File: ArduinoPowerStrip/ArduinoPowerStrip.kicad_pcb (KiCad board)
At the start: 2 copper layers, 53.3 x 68.5 mm, 15 parts, among them P101 Triac1, P102 Triac1, Q101 Q_NPN_BEC, Q102 Q_NPN_BEC, U101 MOC3041M, U102 MOC3041M, U103 TRIAC, U104 TRIAC

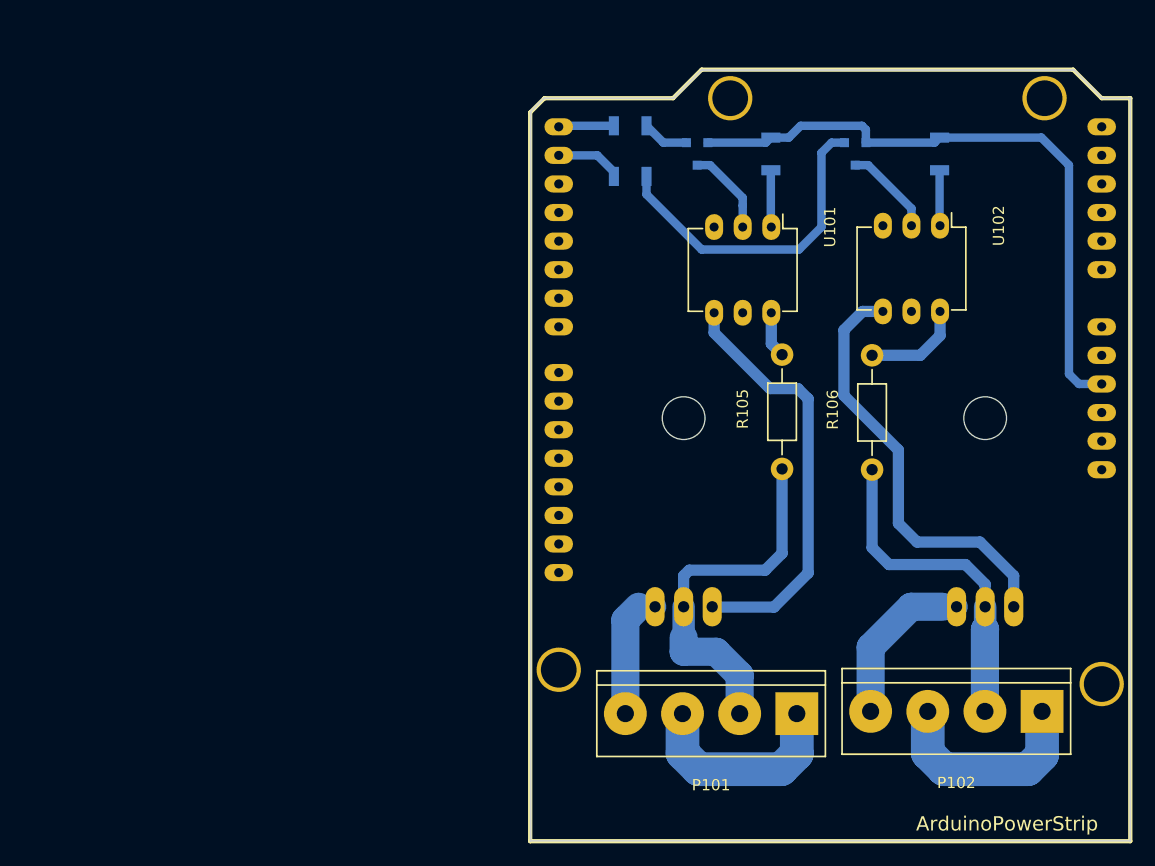
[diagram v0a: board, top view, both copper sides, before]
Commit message: Initial draft of the final board
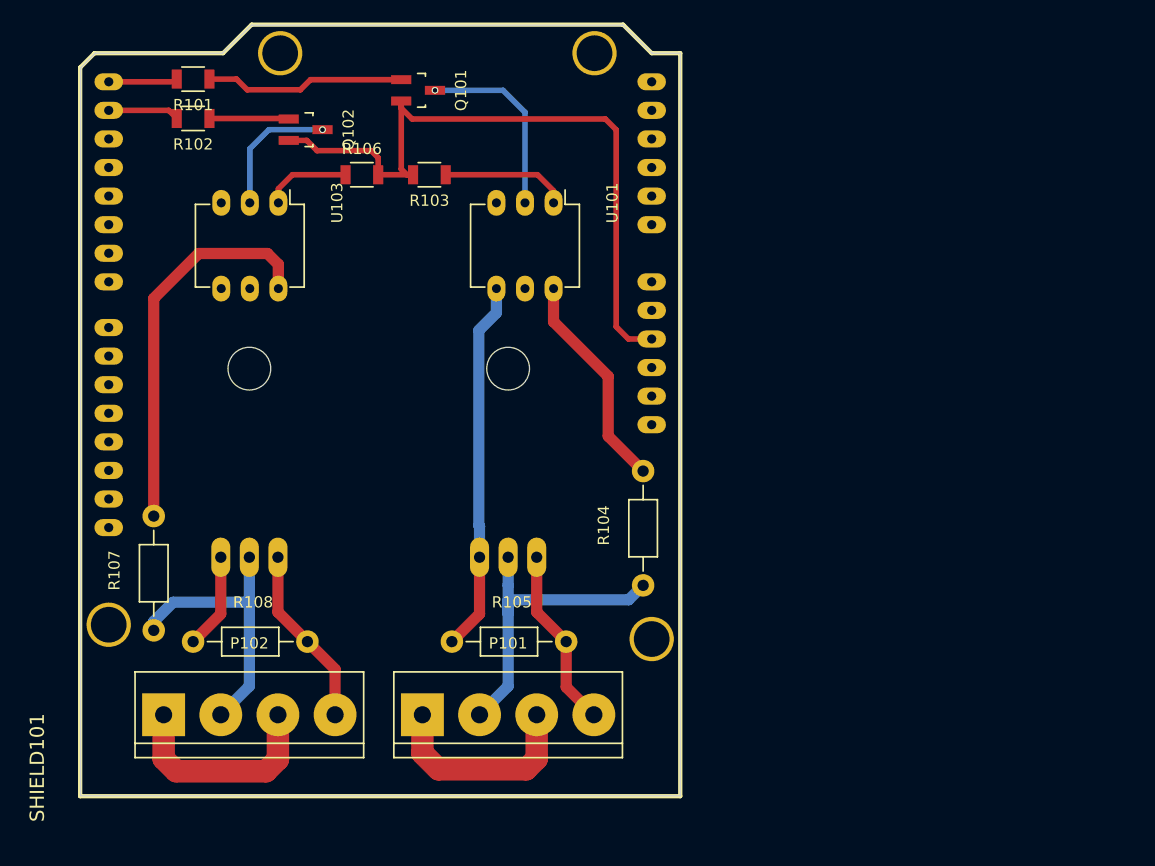
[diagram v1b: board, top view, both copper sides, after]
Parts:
- removed ArduinoPowerStrip: ARDUINO_SHIELD, ArduinoShield:ArduinoShield
- added R107: 361, Resistors_ThroughHole:Resistor_Horizontal_RM10mm, F.Cu at (76.5, 101.5)
- added R108: 331, Resistors_ThroughHole:Resistor_Horizontal_RM10mm, F.Cu at (80.0, 102.5)
- added SHIELD101: ARDUINO_SHIELD, ArduinoShield:ArduinoShield, F.Cu at (123.3, 116.2)
- P101: value Triac1 -> Con1
- P102: value Triac1 -> Con2
- Q101, Q102: value Q_NPN_BEC -> BC847-SOT23; footprint TO_SOT_Packages_SMD:SOT-23 -> TO_SOT_Packages_SMD:SOT-23_Handsoldering; moved to F.Cu
- R101, R102: value R_Small -> 331; moved to F.Cu
- R103: value R_Small -> 131; moved to F.Cu
- R104: value R_Small -> 361; footprint Resistors_SMD:R_1206 -> Resistors_ThroughHole:Resistor_Horizontal_RM10mm; moved to F.Cu
- R105: value R_Small -> 331
- R106: value R_Small -> 131; footprint Resistors_ThroughHole:Resistor_Horizontal_RM10mm -> Resistors_SMD:R_1206
- U102: value MOC3041M -> BTA06-600BW; footprint Housings_DIP:DIP-6_W7.62mm_LongPads -> TO_SOT_Packages_THT:TO-220_Neutral123_Horizontal_LargePads; moved to B.Cu
- U103: value TRIAC -> MOC3041M; footprint TO_SOT_Packages_THT:TO-220_Neutral123_Horizontal_Reverse_LargePads -> Housings_DIP:DIP-6_W7.62mm_LongPads; moved to F.Cu
- U104: value TRIAC -> BTA06-600BW; footprint TO_SOT_Packages_THT:TO-220_Neutral123_Horizontal_Reverse_LargePads -> TO_SOT_Packages_THT:TO-220_Neutral123_Horizontal_LargePads
- moved U104 65.5 mm to (85.0, 95.0)
- moved P102 62.8 mm to (85.0, 109.0), turned to 0 degrees
- moved R106 52.4 mm to (95.0, 61.0), turned to 0 degrees
- moved U103 50.9 mm to (87.6, 63.5), turned to 270 degrees
- moved Q102 48.9 mm to (90.0, 57.0), turned to 270 degrees
- moved U102 48.4 mm to (108.0, 95.0), turned to 180 degrees
- moved R104 46.5 mm to (120.0, 97.5)
- moved R102 39.2 mm to (80.0, 56.0)
- moved R101 39.1 mm to (80.0, 52.5)
- moved R105 33.1 mm to (103.0, 102.5), turned to 0 degrees
- moved R103 30.4 mm to (101.0, 61.0), turned to 180 degrees
- moved Q101 25.4 mm to (100.0, 53.5), turned to 270 degrees
- moved U101 19.5 mm to (112.0, 63.5)
- moved P101 18.0 mm to (108.0, 109.0), turned to 0 degrees
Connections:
- R104 pad 1: Net-(R104-Pad1) -> /Triac1L
- R104 pad 2: /Gnd -> Net-(R104-Pad2)
- R105 pad 1: /Triac1L -> Net-(R105-Pad1)
- R105 pad 2: Net-(R105-Pad2) -> /Triac1O
- R106 pad 1: /Triac2L -> Net-(R106-Pad1)
- R106 pad 2: Net-(R106-Pad2) -> /Gnd
- U101 pad 4: Net-(U101-Pad4) -> Net-(R105-Pad1)
- U101 pad 6: Net-(R105-Pad2) -> Net-(R104-Pad2)
- U102 pad 1: Net-(R104-Pad1) -> /Triac1O
- U102 pad 2: /Q2Out -> /Triac1L
- U102 pad 3: (no net) -> Net-(R105-Pad1)
- U103 pad 1: /Triac1O -> Net-(R106-Pad1)
- U103 pad 2: /Triac1L -> /Q2Out
- U103 pad 3: Net-(U101-Pad4) -> (no net)
- U104 pad 3: Net-(U102-Pad4) -> Net-(R108-Pad1)
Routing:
- net Net-(U102-Pad4): track 38.3 -> 0.00 mm
- net Net-(U101-Pad4): track 37.9 -> 0.00 mm
- net Net-(R107-Pad2): track 0.00 -> 34.6 mm
- net Net-(R105-Pad1): track 0.00 -> 34.0 mm
- net Net-(Q102-Pad1): track 29.0 -> 7.07 mm
- net Net-(R104-Pad2): track 0.00 -> 19.5 mm
- net Net-(Q101-Pad1): track 4.17 -> 17.8 mm
- net /Q1Out: track 7.85 -> 17.2 mm, vias 0 -> 1
- net Net-(R106-Pad2): track 8.91 -> 0.00 mm
- net Net-(R108-Pad1): track 0.00 -> 8.52 mm
- net Net-(R106-Pad1): track 0.00 -> 7.74 mm
- net Net-(R103-Pad1): track 5.07 -> 11.3 mm
- net Net-(R104-Pad1): track 4.95 -> 0.00 mm
- net /Triac1O: track 11.4 -> 16.1 mm
- net /Triac2L: track 29.6 -> 25.0 mm
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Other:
- outline, holes or cut-outs redrawn
- rule pad_to_mask_clearance: 0.2 -> 0
